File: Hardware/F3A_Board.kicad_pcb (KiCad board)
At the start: 2 copper layers, 102.9 x 71.1 mm, 14 parts, among them J1 Conn_01x03, Q1 BC550, Q2 BC550, U1 W25Q64V

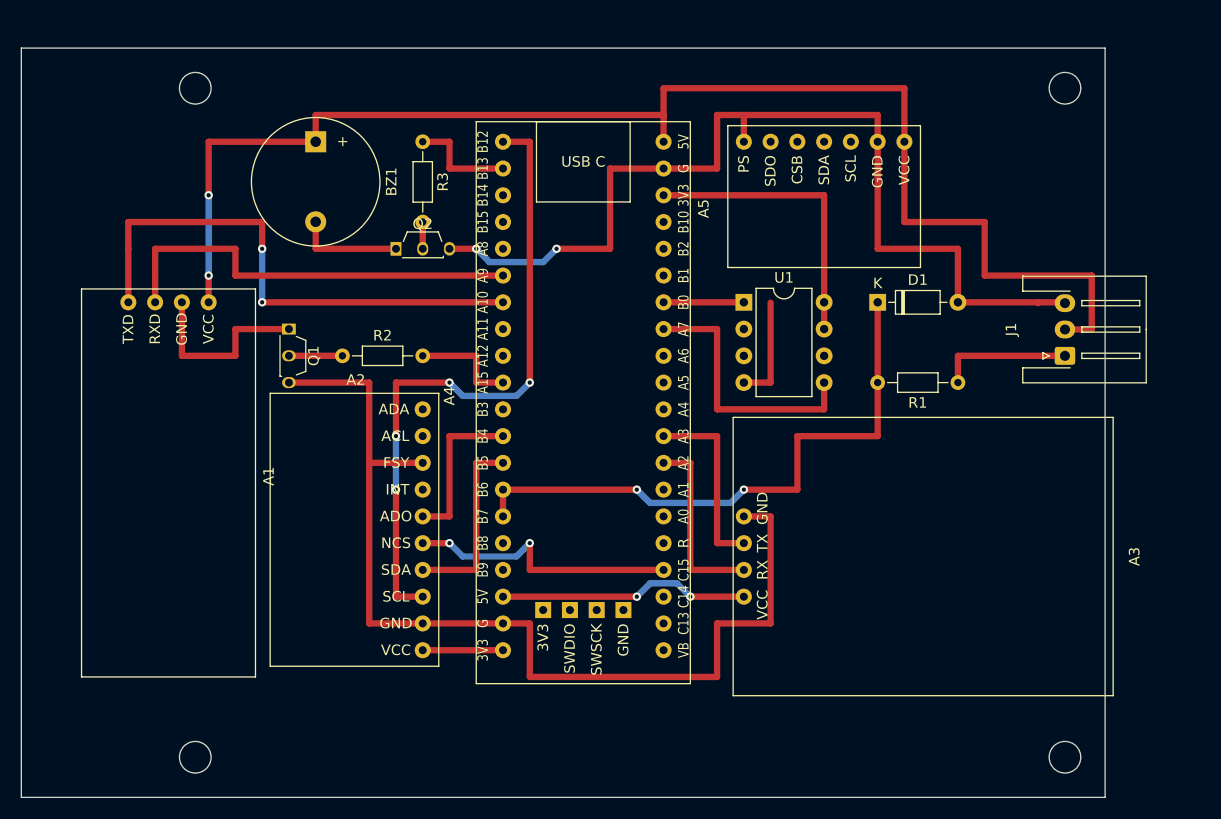
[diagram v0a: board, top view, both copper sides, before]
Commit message: PCBnew updated Created step file
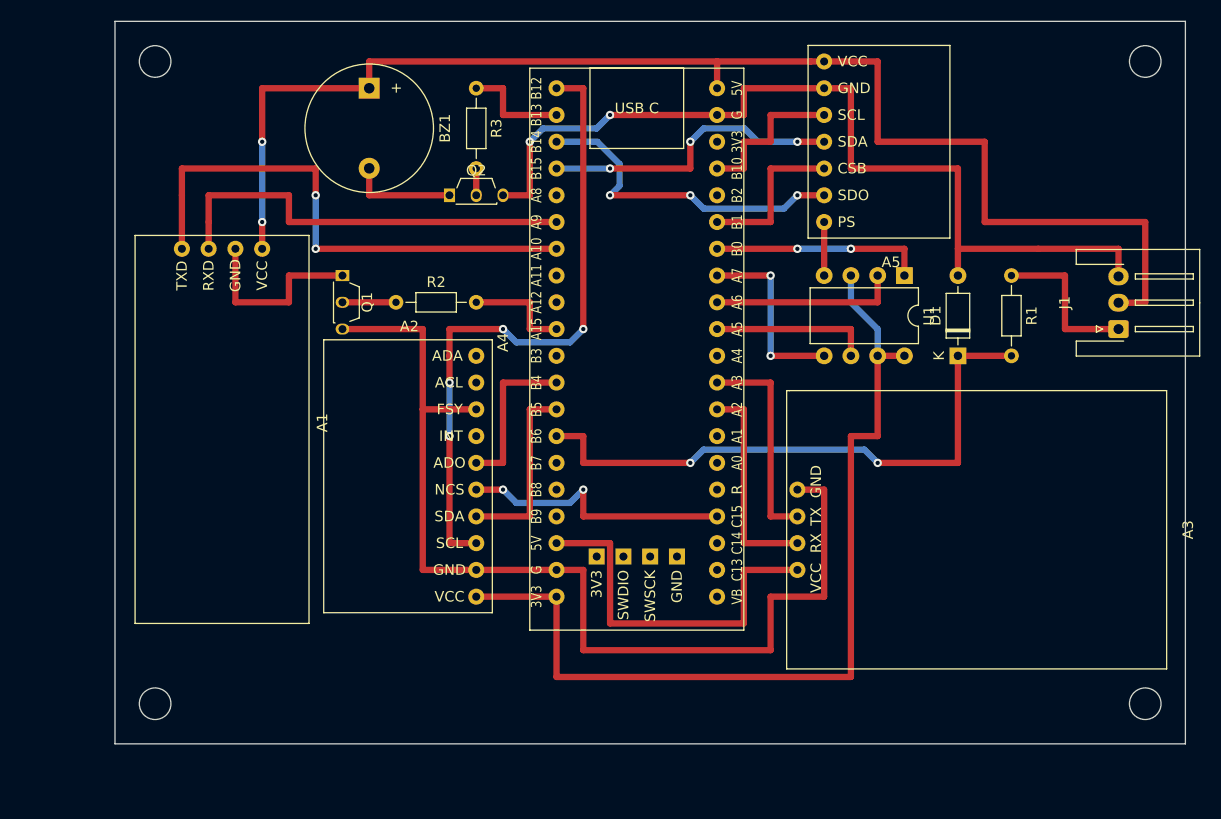
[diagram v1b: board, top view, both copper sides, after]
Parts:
- moved U1 15.5 mm to (198.1, 94.0), turned to 270 degrees
- moved R1 11.4 mm to (208.3, 94.0), turned to 270 degrees
- moved D1 9.16 mm to (203.2, 101.6), turned to 90 degrees
- moved A5 8.98 mm to (196.8, 81.3), turned to 0 degrees
- moved A4 7.18 mm to (172.7, 100.3)
- moved Q1 7.18 mm to (144.8, 94.0)
- moved R2 7.18 mm to (149.9, 96.5)
- moved A1 7.18 mm to (133.3, 108.0)
- moved A2 7.18 mm to (151.1, 113.0)
- moved BZ1 7.18 mm to (147.3, 76.2)
- moved Q2 7.18 mm to (154.9, 86.4)
- moved R3 7.18 mm to (157.5, 76.2)
- moved A3 5.68 mm to (205.7, 118.1)
- moved J1 5.68 mm to (218.4, 99.1)
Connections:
- net Buzzer_PWR renamed Buzzer_PWR_CTRL
- A4 pad 14: PWM_IN -> RC_PWM
- A4 pad 15: PWM_IN -> (no net)
- D1 pad 1: PWM_IN -> RC_PWM
- R1 pad 2: PWM_IN -> RC_PWM
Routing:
- net RC_PWM: track 0.00 -> 56.9 mm, vias 0 -> 2
- net PWM_IN: track 56.9 -> 0.00 mm, vias 2 -> 0
- net +3V3: track 35.6 -> 87.4 mm
- net /SPI2_SDO: track 0.00 -> 31.6 mm, vias 0 -> 3
- net /SPI2_SDI: track 0.00 -> 29.0 mm, vias 0 -> 3
- net /SPI1_SDO: track 0.00 -> 17.8 mm
- net /SPI2_CS: track 0.00 -> 15.2 mm
- net /SPI2_SCL: track 0.00 -> 15.2 mm
- net /SPI1_SCL: track 0.00 -> 15.2 mm
- net /SPI1_CS: track 7.62 -> 20.3 mm, vias 0 -> 2
- net +5V: track 156.1 -> 165.1 mm, vias 4 -> 2
- net GND: track 199.3 -> 191.6 mm
- net /SPI1_SDI: track 25.4 -> 17.8 mm, vias 0 -> 2
- net /UART2_RX: track 17.8 -> 20.3 mm
- net /UART2_TX: track 17.8 -> 20.3 mm
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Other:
- board size 102.9 x 71.1 mm -> 101.6 x 68.6 mm
